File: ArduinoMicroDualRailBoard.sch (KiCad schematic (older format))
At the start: 54 parts, among them J1 Conn_01x20_Male, J2 Screw_Terminal_01x03, J3 Conn_01x20_Male, J4 Conn_01x20_Male, J5 Screw_Terminal_01x03, J6 Conn_01x20_Male, J7 SDS-50J, J8 SDS-50J, U1 L7805, U2 L7815, U3 L7915, U4 ARDUINO_MICRO_SHIELD, U5 74LS126, U6 6N138, U7 240-118ABEH-22, U8 240-118ABEH-22, U9 240-118ABEH-22

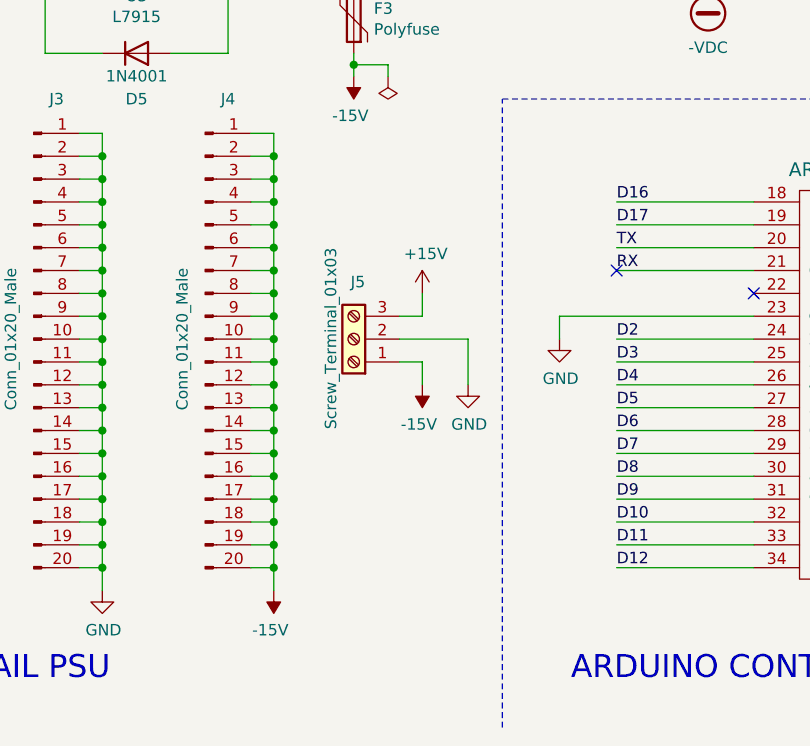
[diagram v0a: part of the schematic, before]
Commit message: PCB layout #2
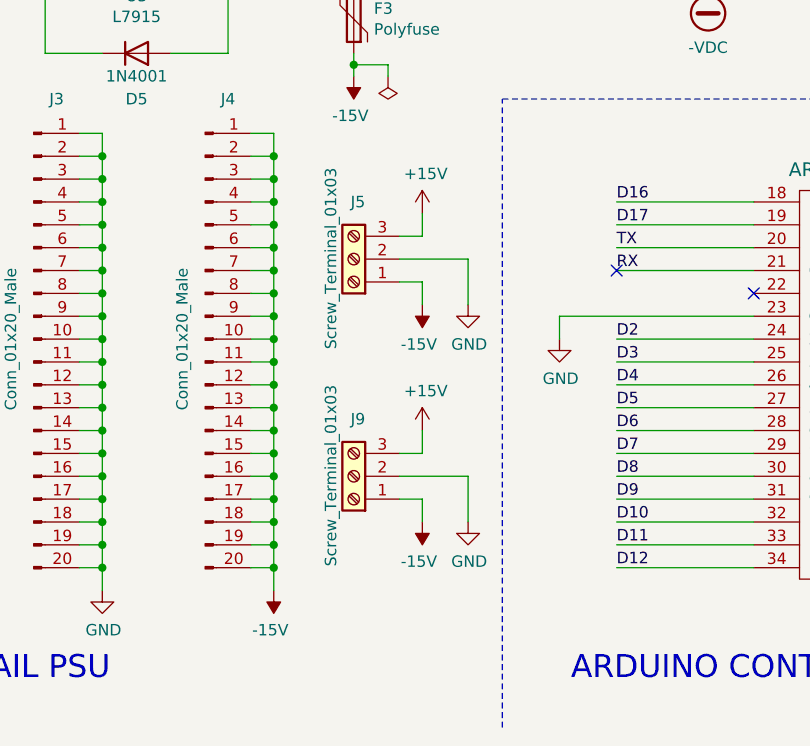
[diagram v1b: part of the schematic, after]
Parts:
- added J9: Screw_Terminal_01x03, TerminalBlock:TerminalBlock_bornier-3_P5.08mm, symbol Connector:Screw_Terminal_01x03
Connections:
- net +15V: now also J9.3 (Pin_3)
- net -15V: now also J9.1 (Pin_1)
- net GND: now also J9.2 (Pin_2)
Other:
- moved on the sheet: J5
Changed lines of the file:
@@
 L Connector:Screw_Terminal_01x03 J5
 U 1 1 60BD4254
-P 3050 6100
-F 0 "J5" H 3000 5850 50  0000 L CNN
-F 1 "Screw_Terminal_01x03" V 3150 5700 50  0000 L CNN
-F 2 "TerminalBlock:TerminalBlock_bornier-3_P5.08mm" H 3050 6100 50  0001 C CNN
-F 3 "~" H 3050 6100 50  0001 C CNN
-	1    3050 6100
+P 3050 5750
+F 0 "J5" H 3000 5500 50  0000 L CNN
+F 1 "Screw_Terminal_01x03" V 3150 5350 50  0000 L CNN
+F 2 "TerminalBlock:TerminalBlock_bornier-3_P5.08mm" H 3050 5750 50  0001 C CNN
+F 3 "~" H 3050 5750 50  0001 C CNN
+	1    3050 5750
 	-1   0    0    1
 $EndComp
@@
 L power:+15V #PWR0131
 U 1 1 60C5B353
-P 3350 5900
-F 0 "#PWR0131" H 3350 5750 50  0001 C CNN
-F 1 "+15V" H 3365 6073 50  0000 C CNN
-F 2 "" H 3350 5900 50  0001 C CNN
-F 3 "" H 3350 5900 50  0001 C CNN
-	1    3350 5900
+P 3350 5550
+F 0 "#PWR0131" H 3350 5400 50  0001 C CNN
+F 1 "+15V" H 3365 5723 50  0000 C CNN
+F 2 "" H 3350 5550 50  0001 C CNN
+F 3 "" H 3350 5550 50  0001 C CNN
+	1    3350 5550
 	1    0    0    -1
 $EndComp
@@
 L power:GND #PWR0132
 U 1 1 60C5D4D3
-P 3550 6300
-F 0 "#PWR0132" H 3550 6050 50  0001 C CNN
-F 1 "GND" H 3555 6127 50  0000 C CNN
-F 2 "" H 3550 6300 50  0001 C CNN
-F 3 "" H 3550 6300 50  0001 C CNN
-	1    3550 6300
+P 3550 5950
+F 0 "#PWR0132" H 3550 5700 50  0001 C CNN
+F 1 "GND" H 3555 5777 50  0000 C CNN
+F 2 "" H 3550 5950 50  0001 C CNN
+F 3 "" H 3550 5950 50  0001 C CNN
+	1    3550 5950
 	1    0    0    -1
 $EndComp
@@
 L power:-15V #PWR0133
 U 1 1 60C5DC2B
-P 3350 6300
-F 0 "#PWR0133" H 3350 6400 50  0001 C CNN
-F 1 "-15V" H 3365 6473 50  0000 C CNN
-F 2 "" H 3350 6300 50  0001 C CNN
-F 3 "" H 3350 6300 50  0001 C CNN
-	1    3350 6300
-	-1   0    0    1
-$EndComp
-Wire Wire Line
-	3250 6200 3350 6200
-Wire Wire Line
-	3350 6200 3350 6300
-Wire Wire Line
-	3250 6100 3550 6100
-Wire Wire Line
-	3550 6100 3550 6300
-Wire Wire Line
-	3250 6000 3350 6000
-Wire Wire Line
-	3350 6000 3350 5900
+P 3350 5950
+F 0 "#PWR0133" H 3350 6050 50  0001 C CNN
+F 1 "-15V" H 3365 6123 50  0000 C CNN
+F 2 "" H 3350 5950 50  0001 C CNN
+F 3 "" H 3350 5950 50  0001 C CNN
+	1    3350 5950
+	-1   0    0    1
+$EndComp
+Wire Wire Line
+	3250 5850 3350 5850
+Wire Wire Line
+	3350 5850 3350 5950
+Wire Wire Line
+	3250 5750 3550 5750
+Wire Wire Line
+	3550 5750 3550 5950
+Wire Wire Line
+	3250 5650 3350 5650
+Wire Wire Line
+	3350 5650 3350 5550
 NoConn ~ 4200 5800
 NoConn ~ 6750 6400
@@
 Wire Wire Line
 	4100 4300 4200 4300
+$Comp
+L Connector:Screw_Terminal_01x03 J9
+U 1 1 5FC225DB
+P 3050 6700
+F 0 "J9" H 3000 6450 50  0000 L CNN
+F 1 "Screw_Terminal_01x03" V 3150 6300 50  0000 L CNN
+F 2 "TerminalBlock:TerminalBlock_bornier-3_P5.08mm" H 3050 6700 50  0001 C CNN
+F 3 "~" H 3050 6700 50  0001 C CNN
+	1    3050 6700
+	-1   0    0    1
+$EndComp
+$Comp
+L power:+15V #PWR01
+U 1 1 5FC225E1
+P 3350 6500
+F 0 "#PWR01" H 3350 6350 50  0001 C CNN
+F 1 "+15V" H 3365 6673 50  0000 C CNN
+F 2 "" H 3350 6500 50  0001 C CNN
+F 3 "" H 3350 6500 50  0001 C CNN
+	1    3350 6500
+	1    0    0    -1
+$EndComp
+$Comp
+L power:GND #PWR03
+U 1 1 5FC225E7
+P 3550 6900
+F 0 "#PWR03" H 3550 6650 50  0001 C CNN
+F 1 "GND" H 3555 6727 50  0000 C CNN
+F 2 "" H 3550 6900 50  0001 C CNN
+F 3 "" H 3550 6900 50  0001 C CNN
+	1    3550 6900
+	1    0    0    -1
+$EndComp
+$Comp
+L power:-15V #PWR02
+U 1 1 5FC225ED
+P 3350 6900
+F 0 "#PWR02" H 3350 7000 50  0001 C CNN
+F 1 "-15V" H 3365 7073 50  0000 C CNN
+F 2 "" H 3350 6900 50  0001 C CNN
+F 3 "" H 3350 6900 50  0001 C CNN
+	1    3350 6900
+	-1   0    0    1
+$EndComp
+Wire Wire Line
+	3250 6800 3350 6800
+Wire Wire Line
+	3350 6800 3350 6900
+Wire Wire Line
+	3250 6700 3550 6700
+Wire Wire Line
+	3550 6700 3550 6900
+Wire Wire Line
+	3250 6600 3350 6600
+Wire Wire Line
+	3350 6600 3350 6500
 $EndSCHEMATC
